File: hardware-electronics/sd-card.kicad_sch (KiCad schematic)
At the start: 39 parts, among them J2 Micro_SD_Card_Det_Hirose_DM3AT, U6 24AA04T-I_OT, U9 USB2244-AEZG-06, Y3 ECS-240-10-47-CKM-TR

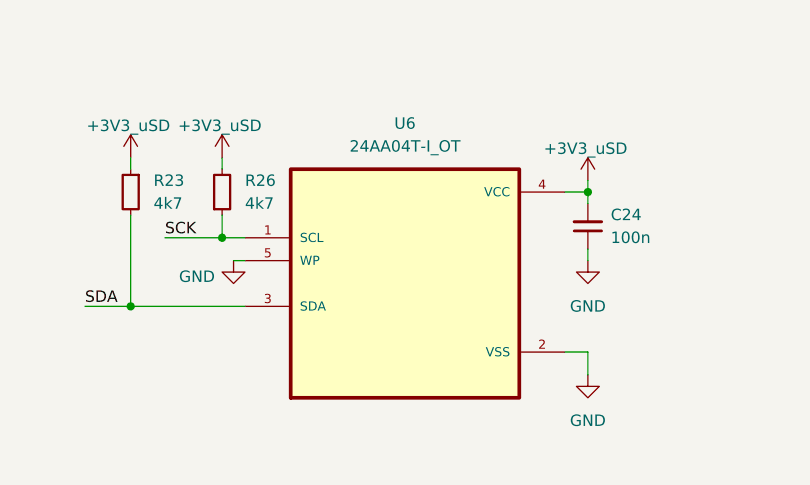
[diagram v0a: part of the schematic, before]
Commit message: SCH update all symbols
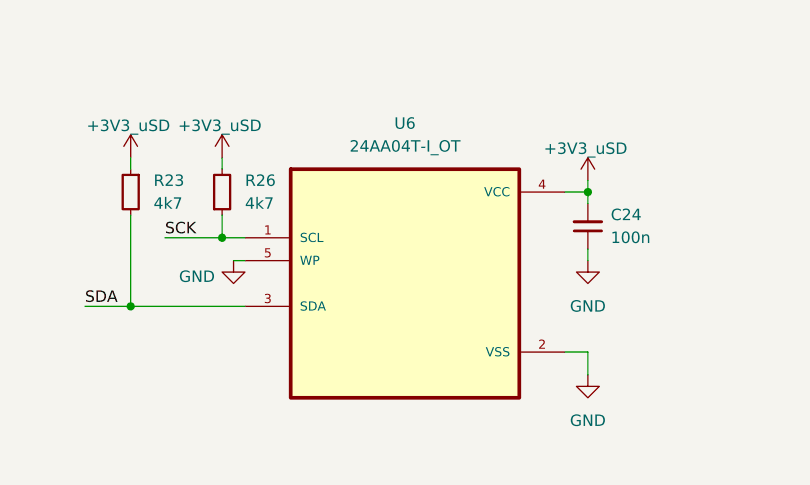
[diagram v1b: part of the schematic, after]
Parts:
- C20, C25: footprint C_4pF_0402:C_0402_1005Metric -> M2SmartHomeFootprints:C_0402
- C24, C27, C29, C31, C33, C35, C39: footprint C_100n_0402:C_0402_1005Metric -> M2SmartHomeFootprints:C_0402
- C26, C28, C30, C32, C34, C36, C37: footprint C_1uF_0402:C_0402_1005Metric -> M2SmartHomeFootprints:C_0201
- C38: footprint C_4u7_0402:C_0402_1005Metric -> M2SmartHomeFootprints:C_0402
- FB5: footprint FB_120R_0603:FB_0603_1608Metric -> M2SmartHomeFootprints:FB_0603
- R21, R22, R24, R25, R32: footprint R_49k9_0402:R_0402_1005Metric -> M2SmartHomeFootprints:R_0402
- R23, R26: footprint R_4k7_0402:R_0402_1005Metric -> M2SmartHomeFootprints:R_0402
- R27, R28: footprint R_500R_0402:R_0402_1005Metric -> M2SmartHomeFootprints:R_0402
- R33, R37, R39: footprint R_10k_0402:R_0402_1005Metric -> M2SmartHomeFootprints:R_0402
- R34: footprint R_0_0402:R_0402_1005Metric -> M2SmartHomeFootprints:R_0402
- R35: footprint R_1M_0402:R_0402_1005Metric -> M2SmartHomeFootprints:R_0402
- R36: footprint R_12k_0402:R_0402_1005Metric -> M2SmartHomeFootprints:R_0402
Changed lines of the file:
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@@
 			)
 		)
-		(property "Footprint" "R_49k9_0402:R_0402_1005Metric"
+		(property "Footprint" "M2SmartHomeFootprints:R_0402"
 			(at 128.27 48.26 0)
 			(effects
@@
 			)
 		)
-		(property "Footprint" "R_49k9_0402:R_0402_1005Metric"
+		(property "Footprint" "M2SmartHomeFootprints:R_0402"
 			(at 123.19 48.26 0)
 			(effects
@@
 			)
 		)
-		(property "Footprint" "C_1uF_0402:C_0402_1005Metric"
+		(property "Footprint" "M2SmartHomeFootprints:C_0201"
 			(at 205.74 86.36 0)
 			(effects
@@
 			)
 		)
-		(property "Footprint" "R_1M_0402:R_0402_1005Metric"
+		(property "Footprint" "M2SmartHomeFootprints:R_0402"
 			(at 60.96 163.83 0)
 			(effects
@@
 			)
 		)
-		(property "Footprint" "R_500R_0402:R_0402_1005Metric"
+		(property "Footprint" "M2SmartHomeFootprints:R_0402"
 			(at 175.26 59.69 0)
 			(effects
@@
 			)
 		)
-		(property "Footprint" "R_49k9_0402:R_0402_1005Metric"
+		(property "Footprint" "M2SmartHomeFootprints:R_0402"
 			(at 118.11 48.26 0)
 			(effects
@@
 			)
 		)
-		(property "Footprint" "C_100n_0402:C_0402_1005Metric"
+		(property "Footprint" "M2SmartHomeFootprints:C_0402"
 			(at 240.03 78.74 0)
 			(effects
@@
 			)
 		)
-		(property "Footprint" "C_4pF_0402:C_0402_1005Metric"
+		(property "Footprint" "M2SmartHomeFootprints:C_0402"
 			(at 46.99 137.16 0)
 			(effects
@@
 			)
 		)
-		(property "Footprint" "C_1uF_0402:C_0402_1005Metric"
+		(property "Footprint" "M2SmartHomeFootprints:C_0201"
 			(at 91.44 60.96 0)
 			(effects
@@
 			)
 		)
-		(property "Footprint" "C_4u7_0402:C_0402_1005Metric"
+		(property "Footprint" "M2SmartHomeFootprints:C_0402"
 			(at 127 87.63 0)
 			(effects
@@
 			)
 		)
-		(property "Footprint" "R_10k_0402:R_0402_1005Metric"
+		(property "Footprint" "M2SmartHomeFootprints:R_0402"
 			(at 93.98 52.07 0)
 			(effects
@@
 			)
 		)
-		(property "Footprint" "C_100n_0402:C_0402_1005Metric"
+		(property "Footprint" "M2SmartHomeFootprints:C_0402"
 			(at 222.25 78.74 0)
 			(effects
@@
 			)
 		)
-		(property "Footprint" "R_4k7_0402:R_0402_1005Metric"
+		(property "Footprint" "M2SmartHomeFootprints:R_0402"
 			(at 96.52 173.99 0)
 			(effects
@@
 			)
 		)
-		(property "Datasheet" ""
+		(property "Datasheet" "https://ww1.microchip.com/downloads/aemDocuments/documents/MPD/ProductDocuments/DataSheets/24AA04-24LC04B-24FC04-4K-I2C-Serial-EEPROM-20001708P.pdf"
 			(at 142.24 166.37 0)
 			(effects
@@
 			)
 		)
-		(property "Footprint" "R_500R_0402:R_0402_1005Metric"
+		(property "Footprint" "M2SmartHomeFootprints:R_0402"
 			(at 111.76 93.98 0)
 			(effects
@@
 			)
 		)
-		(property "Footprint" "R_49k9_0402:R_0402_1005Metric"
+		(property "Footprint" "M2SmartHomeFootprints:R_0402"
 			(at 113.03 48.26 0)
 			(effects
@@
 			)
 		)
-		(property "Footprint" "R_49k9_0402:R_0402_1005Metric"
+		(property "Footprint" "M2SmartHomeFootprints:R_0402"
 			(at 134.62 48.26 0)
 			(effects
@@
 			)
 		)
-		(property "Footprint" "FB_120R_0603:FB_0603_1608Metric"
+		(property "Footprint" "M2SmartHomeFootprints:FB_0603"
 			(at 259.08 101.6 0)
 			(effects
@@
 			)
 		)
-		(property "Footprint" "C_1uF_0402:C_0402_1005Metric"
+		(property "Footprint" "M2SmartHomeFootprints:C_0201"
 			(at 271.78 74.93 0)
 			(effects
@@
 			)
 		)
-		(property "Footprint" "C_1uF_0402:C_0402_1005Metric"
+		(property "Footprint" "M2SmartHomeFootprints:C_0201"
 			(at 288.29 68.58 0)
 			(effects
@@
 			)
 		)
-		(property "Footprint" "C_4pF_0402:C_0402_1005Metric"
+		(property "Footprint" "M2SmartHomeFootprints:C_0402"
 			(at 63.5 137.16 0)
 			(effects
@@
 			)
 		)
-		(property "Footprint" "R_0_0402:R_0402_1005Metric"
+		(property "Footprint" "M2SmartHomeFootprints:R_0402"
 			(at 143.51 86.36 0)
 			(effects
@@
 			)
 		)
-		(property "Footprint" "R_10k_0402:R_0402_1005Metric"
+		(property "Footprint" "M2SmartHomeFootprints:R_0402"
 			(at 138.43 48.26 0)
 			(effects
@@
 			)
 		)
-		(property "Footprint" "R_10k_0402:R_0402_1005Metric"
+		(property "Footprint" "M2SmartHomeFootprints:R_0402"
 			(at 99.06 142.24 0)
 			(effects
@@
 			)
 		)
-		(property "Footprint" "C_100n_0402:C_0402_1005Metric"
+		(property "Footprint" "M2SmartHomeFootprints:C_0402"
 			(at 118.11 87.63 0)
 			(effects
@@
 			)
 		)
-		(property "Footprint" "R_12k_0402:R_0402_1005Metric"
+		(property "Footprint" "M2SmartHomeFootprints:R_0402"
 			(at 191.77 90.17 0)
 			(effects
@@
 			)
 		)
-		(property "Footprint" "C_100n_0402:C_0402_1005Metric"
+		(property "Footprint" "M2SmartHomeFootprints:C_0402"
 			(at 279.4 68.58 0)
 			(effects
@@
 			)
 		)
-		(property "Footprint" "C_100n_0402:C_0402_1005Metric"
+		(property "Footprint" "M2SmartHomeFootprints:C_0402"
 			(at 262.89 74.93 0)
 			(effects
@@
 			)
 		)
-		(property "Footprint" "C_1uF_0402:C_0402_1005Metric"
+		(property "Footprint" "M2SmartHomeFootprints:C_0201"
 			(at 248.92 78.74 0)
 			(effects
@@
 			)
 		)
-		(property "Footprint" "C_100n_0402:C_0402_1005Metric"
+		(property "Footprint" "M2SmartHomeFootprints:C_0402"
 			(at 175.26 142.24 0)
 			(effects
@@
 			)
 		)
-		(property "Footprint" "C_100n_0402:C_0402_1005Metric"
+		(property "Footprint" "M2SmartHomeFootprints:C_0402"
 			(at 196.85 86.36 0)
 			(effects
@@
 			)
 		)
-		(property "Footprint" "C_1uF_0402:C_0402_1005Metric"
+		(property "Footprint" "M2SmartHomeFootprints:C_0201"
 			(at 96.52 154.94 0)
 			(effects
@@
 			)
 		)
-		(property "Footprint" "C_1uF_0402:C_0402_1005Metric"
+		(property "Footprint" "M2SmartHomeFootprints:C_0201"
 			(at 231.14 78.74 0)
 			(effects
@@
 			)
 		)
-		(property "Footprint" "R_4k7_0402:R_0402_1005Metric"
+		(property "Footprint" "M2SmartHomeFootprints:R_0402"
 			(at 137.16 138.43 0)
 			(effects
